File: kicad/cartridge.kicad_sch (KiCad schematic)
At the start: 1 part, among them J1 CommanderX16Expansion

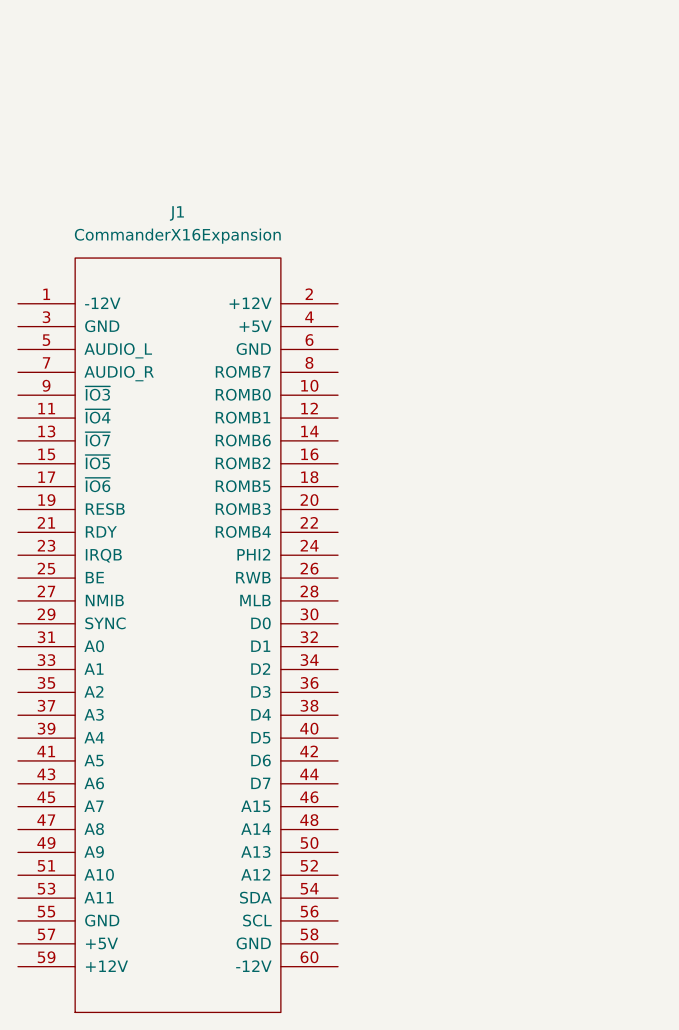
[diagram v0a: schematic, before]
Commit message: second commit
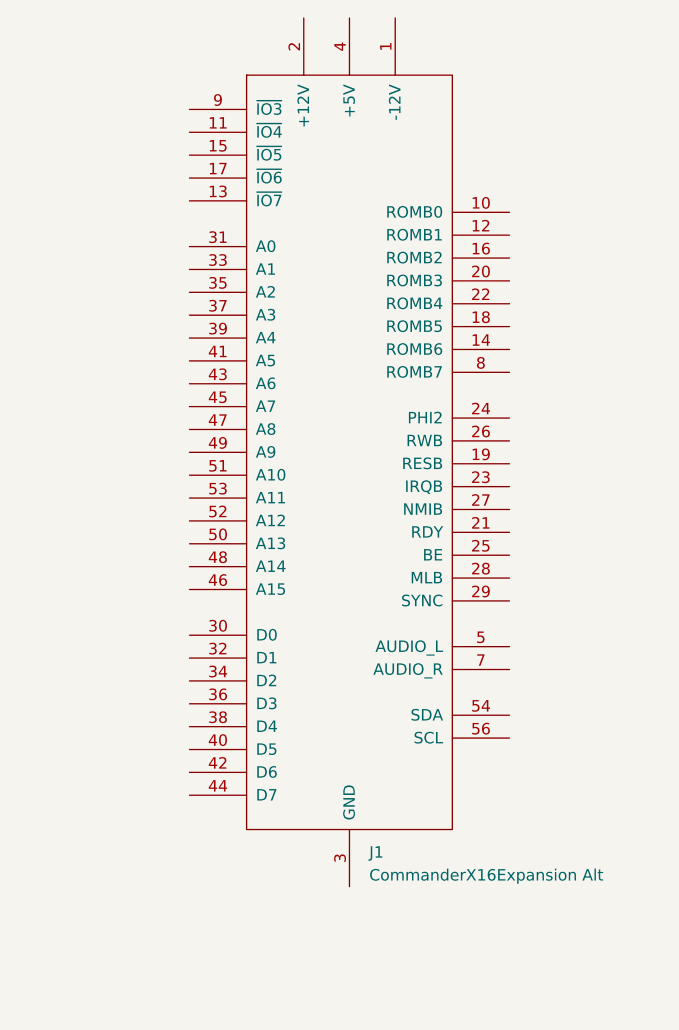
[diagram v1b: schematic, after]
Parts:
- removed J1: CommanderX16Expansion, CommanderX16Expansion:CommanderX16Expansion, symbol CommanderX16Expansion:CommanderX16Expansion
- added J1: CommanderX16Expansion Alt, CommanderX16Expansion:CommanderX16Expansion, symbol CommanderX16Expansion:CommanderX16Expansion Alt
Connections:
- new net: J1.1 (-12V), J1.60 (-12V)
- new net: J1.2 (+12V), J1.59 (+12V)
- new net: J1.3 (GND), J1.55 (GND), J1.58 (GND), J1.6 (GND)
- new net: J1.4 (+5V), J1.57 (+5V)
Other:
- title: (none) -> CX16 Open Cartridge
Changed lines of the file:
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@@
 (kicad_sch (version 20230121) (generator eeschema)
-  (paper "A4")
-  (symbol (lib_id "CommanderX16Expansion:CommanderX16Expansion") (at 137.16 96.52 0) (unit 1)
+  (paper "USLetter" portrait)
+  (title_block
+    (title "CX16 Open Cartridge")
+    (date "2023-12-11")
+    (rev "v0.1.0-alpha")
+    (comment 2 "creativecommons.org/licenses/by/4.0/")
+    (comment 3 "License: CC BY 4.0")
+    (comment 4 "Author: connorwillchris")
+  )
+  (symbol (lib_id "CommanderX16Expansion:CommanderX16Expansion Alt") (at 156.21 76.2 0) (unit 1)
     (in_bom no) (on_board yes) (dnp no) (fields_autoplaced)
-    (property "Reference" "J1" (at 137.16 49.53 0)
-      (effects (font (size 1.27 1.27)))
+    (property "Reference" "J1" (at 158.4041 120.65 0)
+      (effects (font (size 1.27 1.27)) (justify left))
     )
-    (property "Value" "CommanderX16Expansion" (at 137.16 52.07 0)
-      (effects (font (size 1.27 1.27)))
+    (property "Value" "CommanderX16Expansion Alt" (at 158.4041 123.19 0)
+      (effects (font (size 1.27 1.27)) (justify left))
     )
-    (property "Footprint" "CommanderX16Expansion:CommanderX16Expansion" (at 137.16 96.52 0)
+    (property "Footprint" "CommanderX16Expansion:CommanderX16Expansion" (at 156.21 76.2 0)
       (effects (font (size 1.27 1.27)) hide)
     )
-    (property "Datasheet" "https://github.com/x16community/x16-docs" (at 137.16 96.52 0)
+    (property "Datasheet" "https://github.com/x16community/x16-docs" (at 156.21 76.2 0)
       (effects (font (size 1.27 1.27)) hide)
     )
+    (pin "27")
+    (pin "20")
+    (pin "30")
+    (pin "3")
+    (pin "29")
+    (pin "15")
+    (pin "2")
+    (pin "21")
+    (pin "23")
+    (pin "22")
+    (pin "10")
+    (pin "1")
+    (pin "13")
+    (pin "12")
+    (pin "11")
+    (pin "14")
+    (pin "31")
+    (pin "24")
+    (pin "26")
+    (pin "41")
+    (pin "42")
+    (pin "43")
+    (pin "44")
     (pin "45")
     (pin "46")
     (pin "47")
     (pin "48")
+    (pin "28")
+    (pin "35")
+    (pin "36")
+    (pin "37")
+    (pin "16")
+    (pin "17")
+    (pin "56")
+    (pin "57")
+    (pin "58")
+    (pin "59")
+    (pin "6")
+    (pin "60")
+    (pin "7")
+    (pin "8")
+    (pin "9")
+    (pin "19")
+    (pin "25")
+    (pin "18")
     (pin "49")
     (pin "5")
@@
     (pin "54")
     (pin "55")
-    (pin "56")
-    (pin "57")
-    (pin "58")
-    (pin "59")
-    (pin "22")
-    (pin "24")
-    (pin "25")
-    (pin "18")
-    (pin "19")
-    (pin "2")
-    (pin "16")
-    (pin "21")
-    (pin "28")
-    (pin "29")
-    (pin "3")
-    (pin "30")
-    (pin "31")
-    (pin "26")
-    (pin "27")
-    (pin "32")
     (pin "33")
     (pin "34")
-    (pin "35")
-    (pin "36")
-    (pin "37")
     (pin "38")
     (pin "39")
     (pin "4")
     (pin "40")
-    (pin "41")
-    (pin "42")
-    (pin "43")
-    (pin "44")
-    (pin "11")
-    (pin "15")
-    (pin "12")
-    (pin "14")
-    (pin "10")
-    (pin "1")
-    (pin "17")
-    (pin "20")
-    (pin "13")
-    (pin "23")
-    (pin "6")
-    (pin "60")
-    (pin "7")
-    (pin "8")
-    (pin "9")
+    (pin "32")
     (instances
       (project "cartridge"
